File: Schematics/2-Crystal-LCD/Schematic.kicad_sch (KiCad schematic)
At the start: 4 parts, among them U1 YAAJ_BluePill_Part_Like_SWD_B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

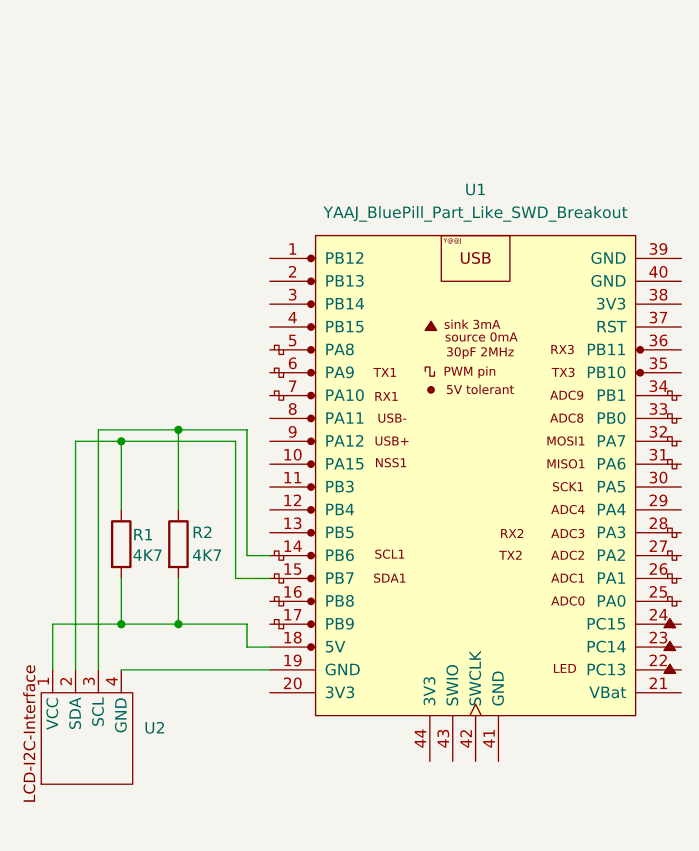
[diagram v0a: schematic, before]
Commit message: update schematics
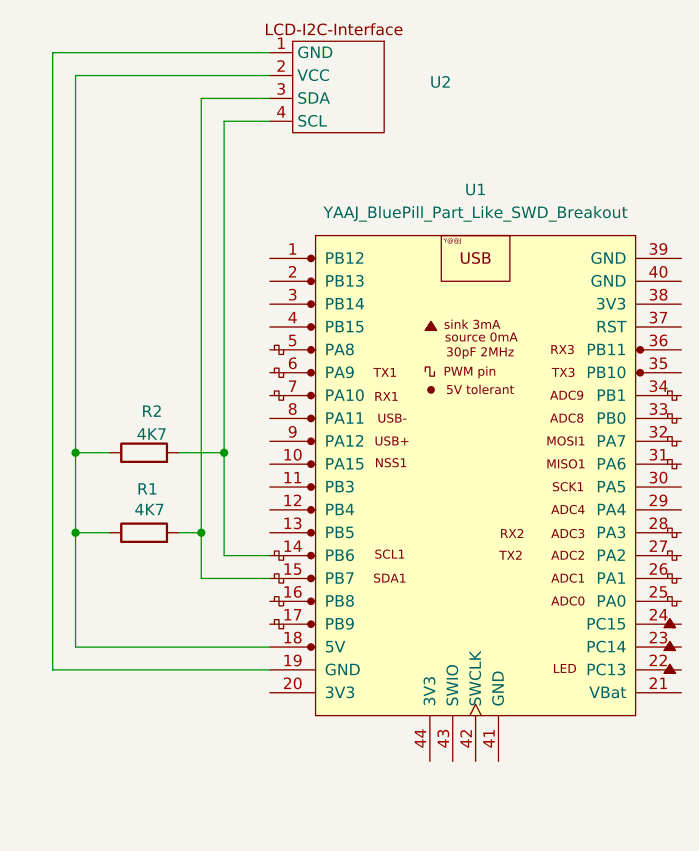
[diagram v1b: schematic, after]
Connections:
- net at R1.1, U2.2 (VCC): now also R2.1, U1.18 (5V); no longer U1.15 (PB7)
- net at U2.4 (SCL): now also R2.2, U1.14 (PB6); no longer U1.19 (GND)
- new net: R1.2, U1.15 (PB7), U2.3 (SDA)
- new net: U1.19 (GND), U2.1 (GND)
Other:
- moved on the sheet: R1, R2
